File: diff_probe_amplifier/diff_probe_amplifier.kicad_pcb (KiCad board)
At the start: 4 copper layers, 25.6 x 37 mm, 86 parts, among them J1 Triax_inner, J2 Triax_outer, J3 Spring+S, J4 Spring+G, J5 Spring-G, J6 Spring-S, J7 IN+, J8 IN-, SW1 GAIN, SW2 Calibrate, U1 R1283K001C, U2 OPA659, U3 OPA659, U4 OPA659, U5 MIC5225-5.0YM5, U6 ATtiny826-M, U7 MCP4451

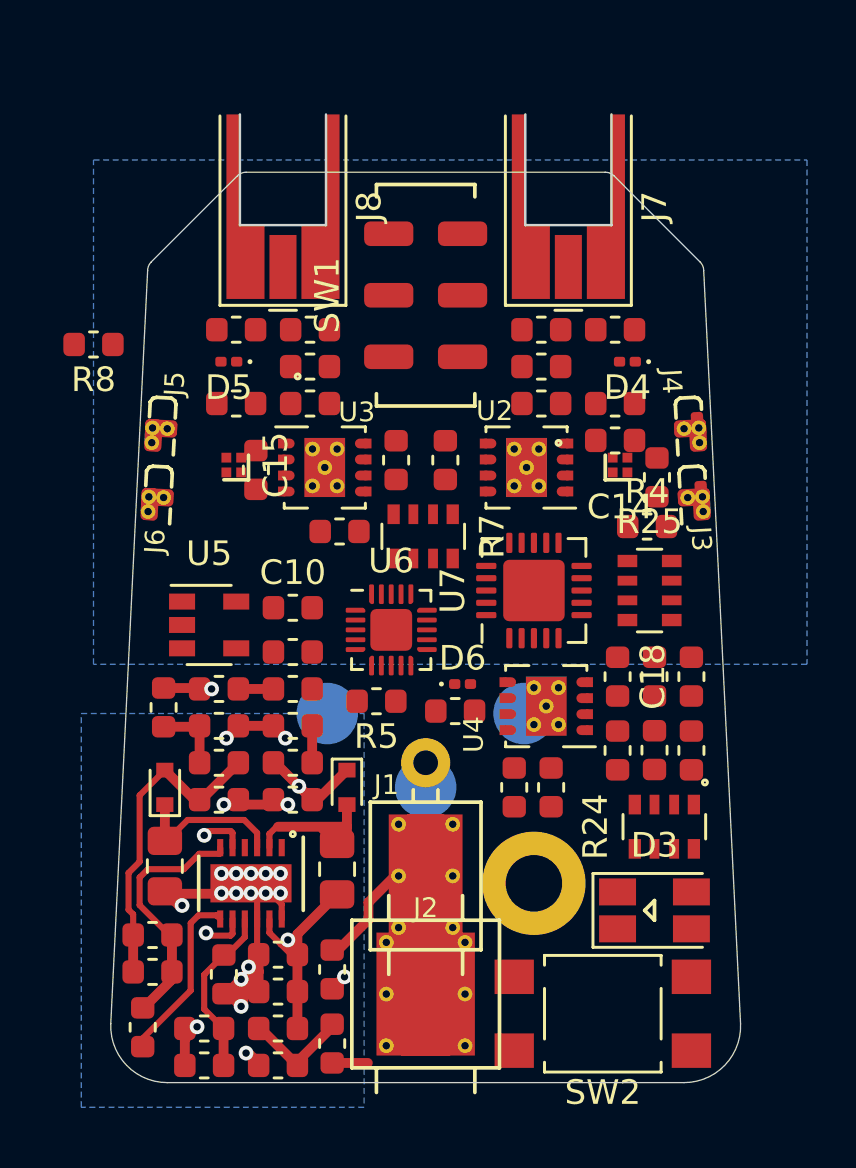
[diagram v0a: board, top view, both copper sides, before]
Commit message: Revision 4
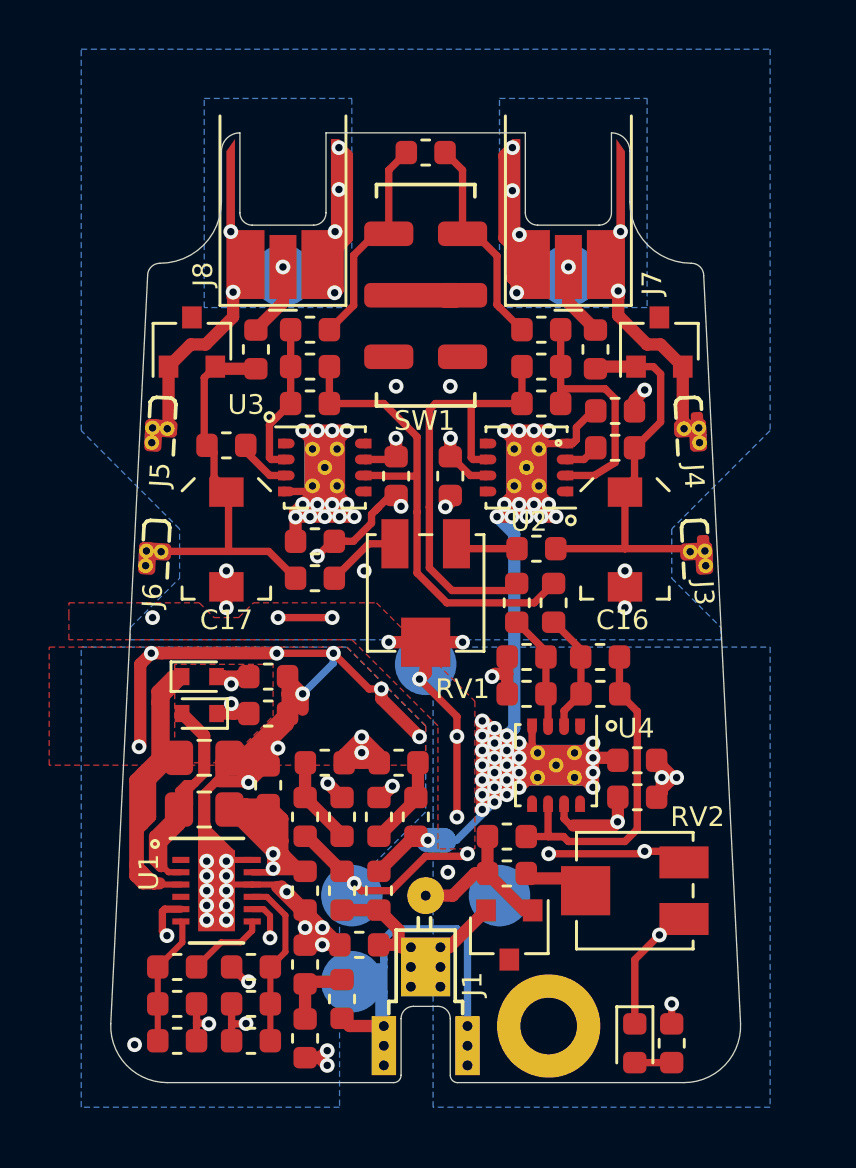
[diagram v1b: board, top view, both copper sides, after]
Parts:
- removed C10: 10µF, Capacitor_SMD:C_0603_1608Metric
- removed C14, C15: LXRW, oscilloscope-probes:LXRW
- removed J2: Triax_outer, oscilloscope-probes:TRIAX_OUTER_3MM
- removed R24, R25: 6.8k, Resistor_SMD:R_Array_Convex_4x0603
- removed R5: 5.1k, Resistor_SMD:R_0603_1608Metric
- removed SW2: Calibrate, Button_Switch_SMD:SW_SPST_TL3305A
- removed U5: MIC5225-5.0YM5, Package_TO_SOT_SMD:SOT-23-5
- removed U6: ATtiny826-M, Package_DFN_QFN:VQFN-20-1EP_3x3mm_P0.4mm_EP1.7x1.7mm
- removed U7: MCP4451, Package_DFN_QFN:QFN-20-1EP_4x4mm_P0.5mm_EP2.5x2.5mm
- added C16: 4.5-20pF, oscilloscope-probes:C_Trimmer_Knowles_JZ_JR, F.Cu at (92.1, 129.9)
- added C17: 4.5-20pF, oscilloscope-probes:C_Trimmer_Knowles_JZ_JR, F.Cu at (75.9, 129.9)
- added RV1: 25k, Potentiometer_SMD:Potentiometer_Bourns_3314J_Vertical, F.Cu at (84.0, 132.1)
- added RV2: 25k, Potentiometer_SMD:Potentiometer_Bourns_3314J_Vertical, F.Cu at (92.5, 144.2)
- added TP7: IN+, TestPoint:TestPoint_Pad_D2.5mm, B.Cu at (89.8, 119.2)
- added TP8: IN-, TestPoint:TestPoint_Pad_D2.5mm, B.Cu at (78.2, 119.2)
- D1, D2: value NSR05T30 -> SBR1A20
- D3: value APBD3224 -> RED; footprint oscilloscope-probes:APBD3224 -> LED_SMD:LED_0603_1608Metric
- D4, D5, D6: value PESD5V0H1BSF -> PESD5V0X1B; footprint Diode_SMD:D_0201_0603Metric -> Package_TO_SOT_SMD:SOT-23
- J1: value Triax_inner -> Conn_Triaxial; footprint oscilloscope-probes:COAX_2MM -> oscilloscope-probes:TRIAX_SOLDER
- J7, J8: footprint Connector_Coaxial:MMCX_Molex_73415-0961_Horizontal_1.6mm-PCB -> oscilloscope-probes:MMCX_Molex_73415-0961_Horizontal_1.6mm-PCB
- L1, L2, L9: value MMZ1608B601 -> BLM18KG102
- R4: value 5.1k -> 22k
- R7: value 6.8k -> 1k; footprint Resistor_SMD:R_Array_Convex_4x0603 -> Resistor_SMD:R_0603_1608Metric
- R8: value 30k -> 5.1k
- moved R8 36.9 mm to (94.0, 150.4), turned to 90 degrees
- moved R4 17.7 mm to (84.0, 114.2), turned to 180 degrees
- moved R7 14.1 mm to (87.3, 143.5), turned to 180 degrees
- moved L8 11.2 mm to (83.6, 141.2), turned to 270 degrees
- moved C13 10.5 mm to (82.1, 144.2), turned to 270 degrees
- moved D6 10.4 mm to (87.4, 146.0), turned to 270 degrees
- moved C12 8.44 mm to (80.6, 144.2), turned to 270 degrees
- moved R19 8.21 mm to (89.2, 132.5), turned to 270 degrees
- moved R18 7.71 mm to (87.7, 132.5)
- moved TP2 7.47 mm to (81.0, 144.4)
- moved TP3 7.47 mm to (87.0, 144.4)
- moved C9 7.45 mm to (82.9, 139.0), turned to 180 degrees
- moved C3 6.90 mm to (77.6, 139.9), turned to 90 degrees
- moved L6 6.86 mm to (82.1, 141.2), turned to 270 degrees
- moved L7 6.72 mm to (79.1, 141.2), turned to 270 degrees
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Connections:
- D3 pad 1: Net-(D3-Pad1) -> -6V
- R4 pad 1: Net-(R4-Pad1) -> Net-(R16-Pad2)
- R4 pad 2: +5VA -> Net-(R17-Pad2)
- R7 pad 1: Net-(R12-Pad2) -> /OFFSET_TRIM
- R7 pad 2: /DC_CMRR2 -> /OUT
- R8 pad 1: Net-(C1-Pad1) -> Net-(D3-Pad2)
- R8 pad 2: Net-(C11-Pad2) -> GNDA
- SW1 pad 1: Net-(SW1-Pad1) -> Net-(R17-Pad2)
- SW1 pad 2: Net-(R17-Pad2) -> Net-(R16-Pad2)
- SW1 pad 3: Net-(R16-Pad2) -> (no net)
- SW1 pad 4: Net-(SW1-Pad4) -> (no net)
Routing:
- net GNDA: track 5.90 -> 118.1 mm, vias 0 -> 35
- net -6V: track 16.9 -> 93.6 mm, vias 1 -> 54
- net GND: track 31.9 -> 103.3 mm, vias 20 -> 27
- net +6V: track 0.00 -> 50.7 mm, vias 0 -> 8
- net Net-(C26-Pad1): track 20.7 -> 62.3 mm, vias 3 -> 6
- net Net-(C11-Pad1): track 0.00 -> 19.5 mm
- net +5V: track 1.45 -> 20.9 mm
- net Net-(D1-Pad1): track 6.55 -> 25.8 mm
- net Net-(C1-Pad2): track 0.00 -> 18.8 mm
- net Net-(C5-Pad1): track 13.0 -> 30.7 mm, vias 0 -> 3
- net /IN-: track 0.00 -> 16.3 mm
- net /IN+: track 0.00 -> 16.3 mm
- net Net-(C19-Pad1): track 0.00 -> 14.1 mm
- net Net-(C1-Pad1): track 0.00 -> 11.4 mm
- net Net-(R17-Pad2): track 0.00 -> 8.82 mm
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- added copper zone on In1.Cu, net -6V
- added copper zone on In2.Cu, net -6V
- added copper zone on F.Cu, net GND
- added copper zone on In1.Cu, net GND
- added copper zone on B.Cu, net GNDA
- added copper zone on F.Cu, net GNDA
- added copper zone on In1.Cu, net GNDA
- added copper zone on In2.Cu, net GNDA
- removed copper zone on In2.Cu, net GND
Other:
- board size 25.6 x 37 mm -> 25.6 x 38.6 mm
- board text added: "DEDP-100 Rev 4, 8/2021"
- board text added: "https://github.com/devEmbedded/differential_probe"
- board text removed: "DEDP-100 Rev 3, 6/2021"
